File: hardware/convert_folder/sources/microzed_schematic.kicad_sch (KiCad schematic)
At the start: 15 parts, among them J19 87832-1420, J4 87832-1420

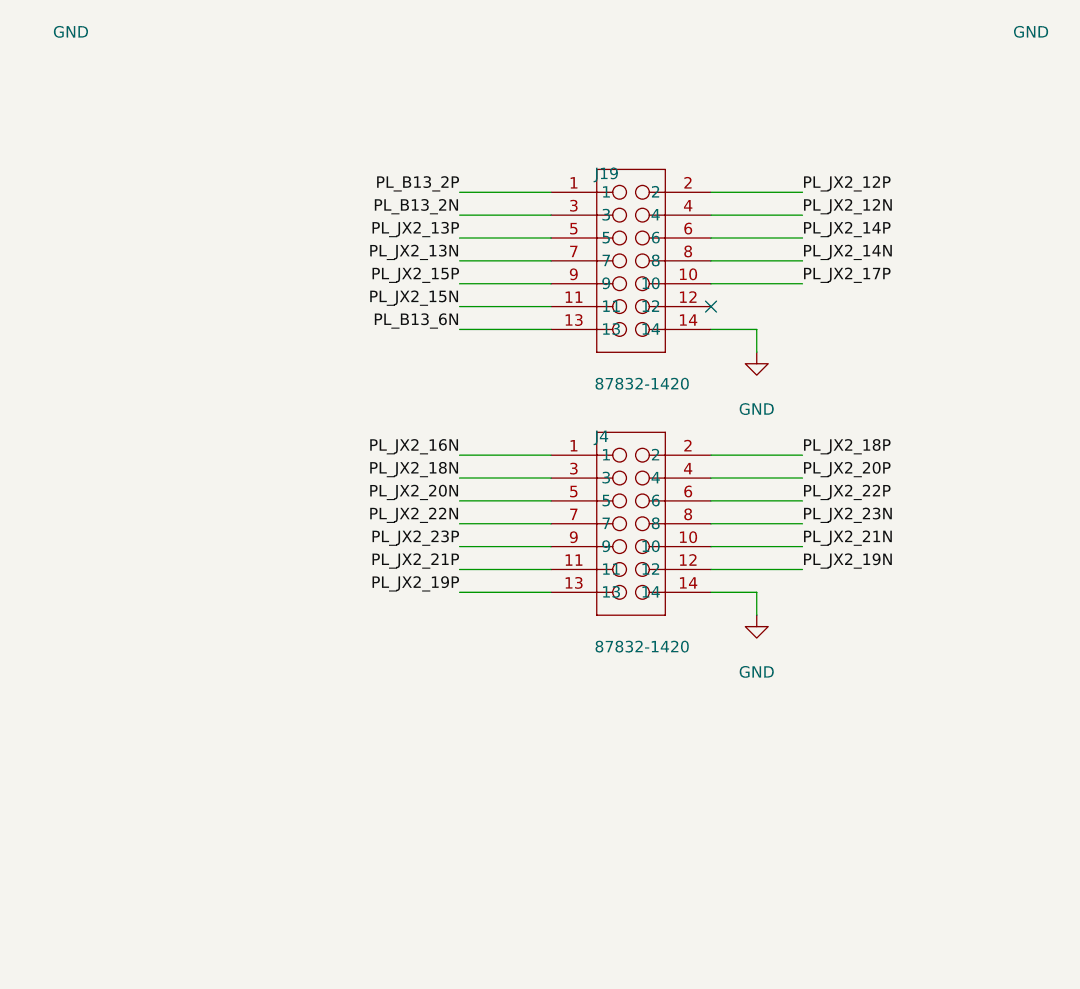
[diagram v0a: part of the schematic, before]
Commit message: fix: fix position of components and signals routing
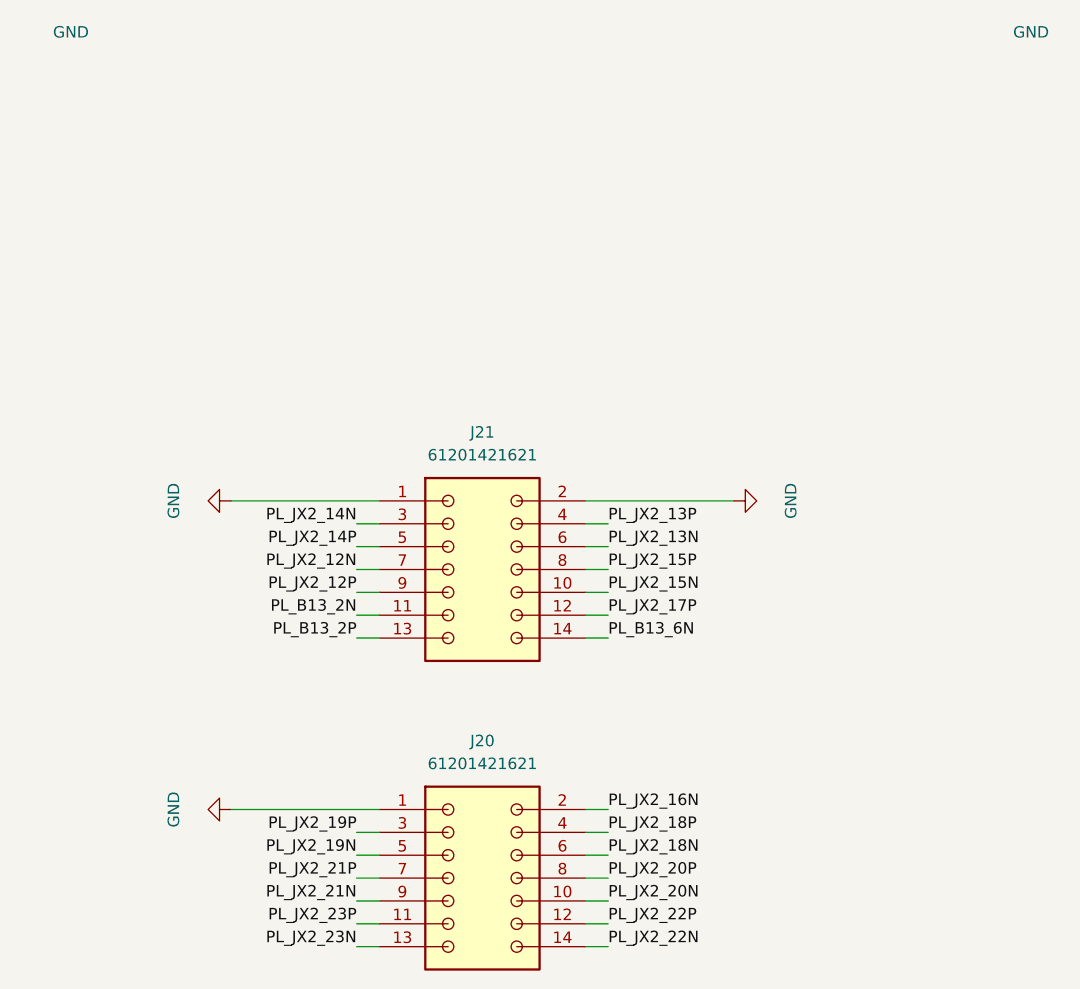
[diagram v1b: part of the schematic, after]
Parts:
- removed J19, J4: 87832-1420, altium_import:SAMTEC_TSW-107-05-F-D, symbol altium_import:root_0_87832-1420_flatsat_platform_2.SchLib
- added J20, J21: 61201421621, lib:61201421621, symbol lib:61201421621
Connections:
- net GND: now also J20.1, J21.1, J21.2
- net PL_B13_2N: now also J21.11
- net PL_B13_2P: now also J21.13
- net PL_B13_6N: now also J21.14
- net PL_JX2_12N: now also J21.7
- net PL_JX2_12P: now also J21.9
- net PL_JX2_13N: now also J21.6
- net PL_JX2_13P: now also J21.4
- net PL_JX2_14N: now also J21.3
- net PL_JX2_14P: now also J21.5
- net PL_JX2_15N: now also J21.10
- net PL_JX2_15P: now also J21.8
- net PL_JX2_16N: now also J20.2
- net PL_JX2_18N: now also J20.6
- net PL_JX2_18P: now also J20.4
- net PL_JX2_19N: now also J20.5
- net PL_JX2_19P: now also J20.3
- net PL_JX2_20N: now also J20.10
- net PL_JX2_20P: now also J20.8
- net PL_JX2_21N: now also J20.9
- net PL_JX2_21P: now also J20.7
- net PL_JX2_22N: now also J20.14
- net PL_JX2_22P: now also J20.12
- net PL_JX2_23N: now also J20.13
- net PL_JX2_23P: now also J20.11
- net at SOM1.JX2-68 (JX2_LVDS_17_P): now also J21.12
- no-connect marks 15 -> 14
